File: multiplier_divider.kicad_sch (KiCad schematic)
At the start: 3 parts, among them J31 Output, J32 Output, SW5 Chain

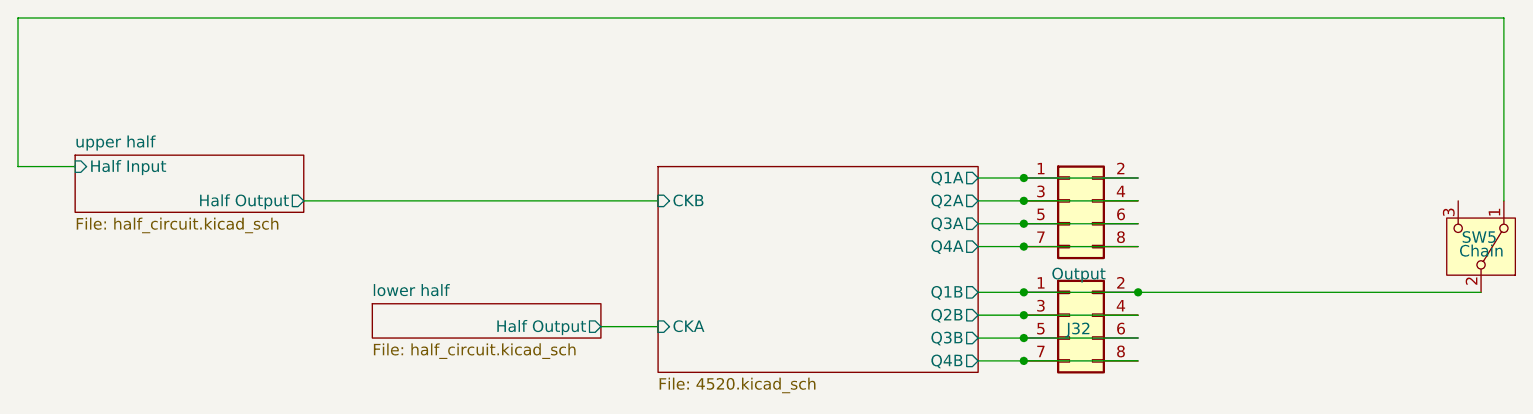
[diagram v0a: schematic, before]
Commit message: wip assemblying everything
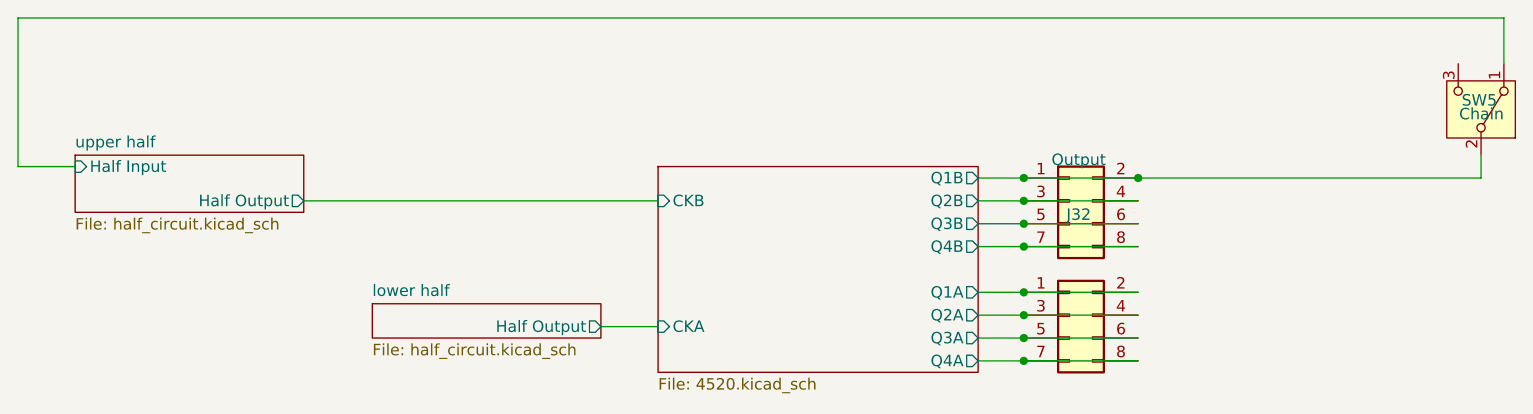
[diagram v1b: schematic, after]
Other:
- moved on the sheet: J32, SW5
